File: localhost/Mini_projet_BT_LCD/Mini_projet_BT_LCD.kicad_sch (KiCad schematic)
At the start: 9 parts

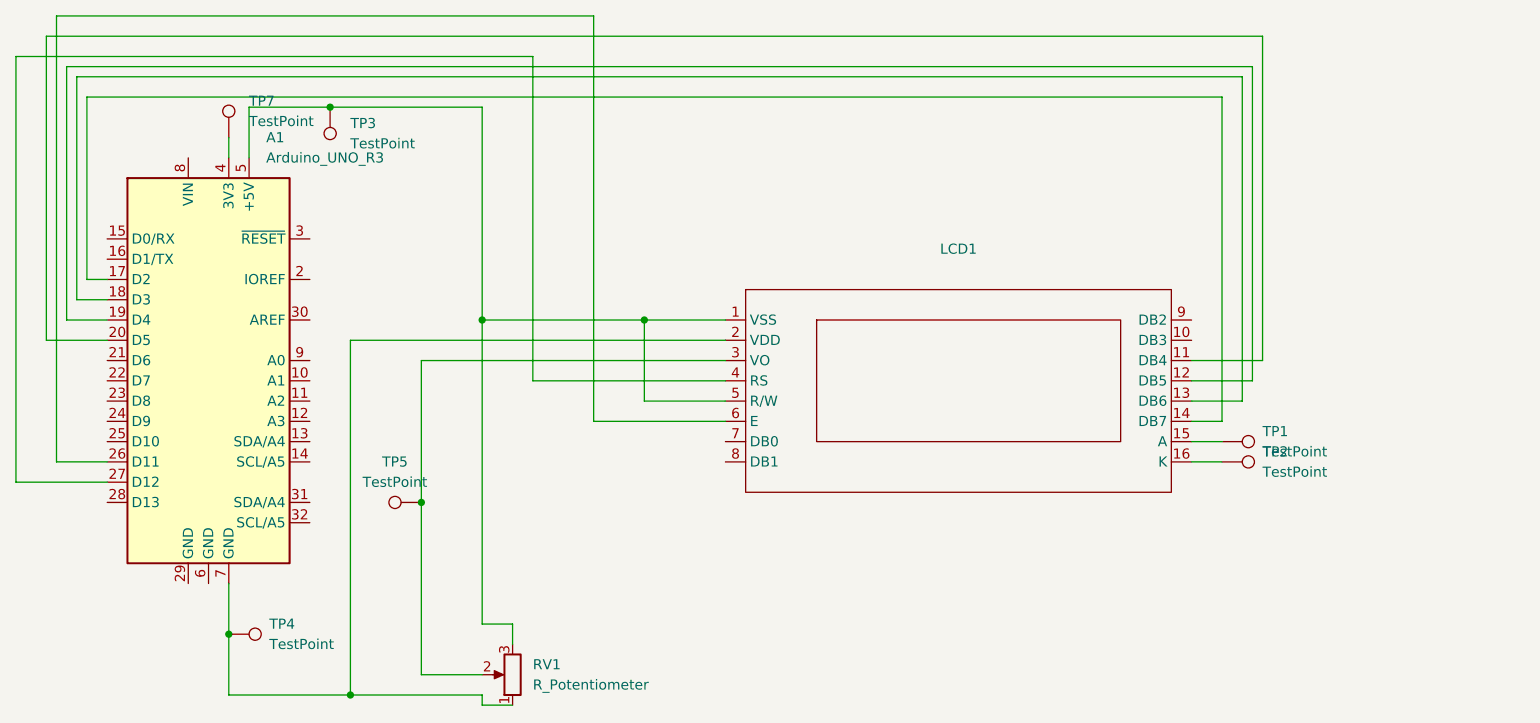
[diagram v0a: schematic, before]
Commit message: Mise à jour 2
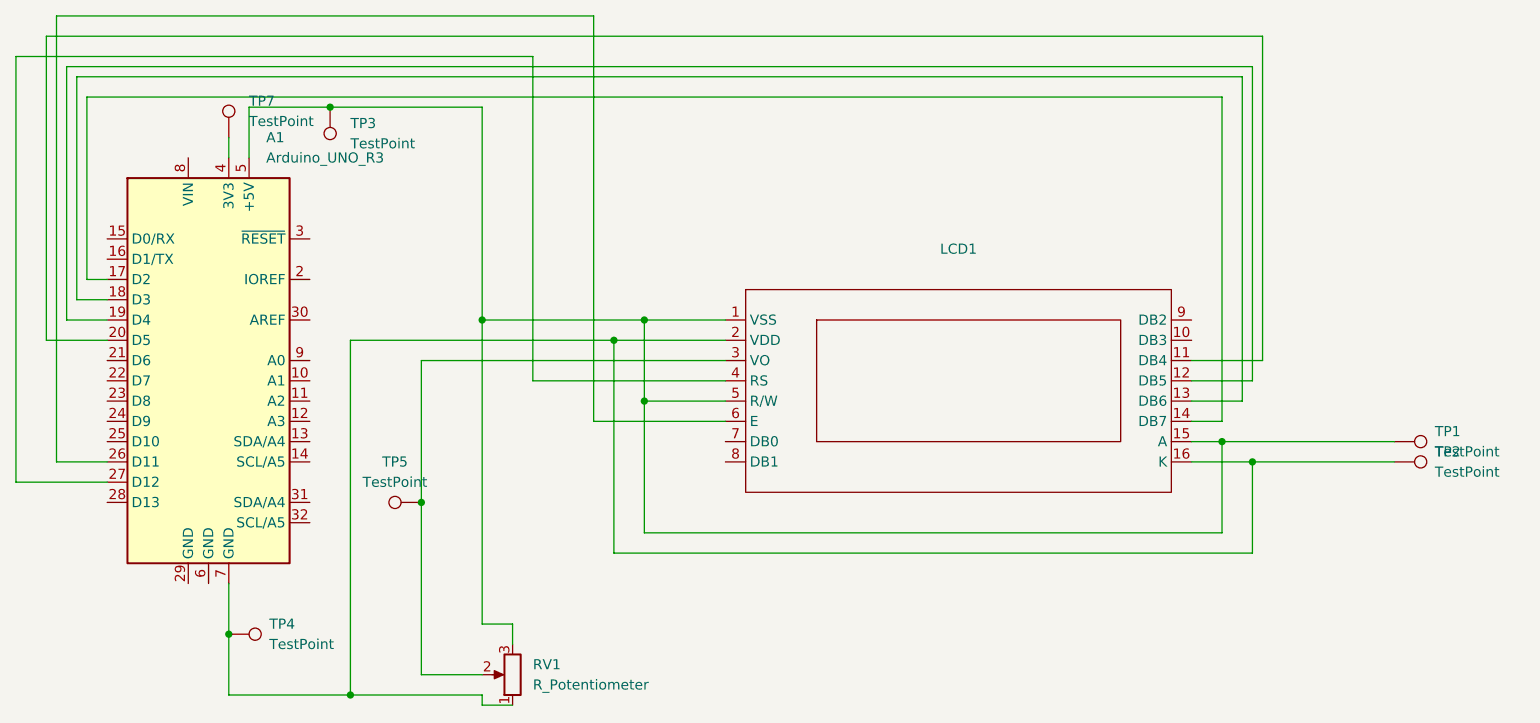
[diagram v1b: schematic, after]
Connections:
- net at A1.7 (GND), LCD1.2 (VDD), RV1.1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: now also LCD1.16 (K), TP2.1
- net at A1.5 (+5V), LCD1.1 (VSS), LCD1.5 (R/W)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: now also LCD1.15 (A), TP1.1
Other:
- moved on the sheet: TP1, TP2
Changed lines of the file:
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@@
+	)
+	(junction
+		(at 193.04 85.09)
+		(diameter 0)
+		(color 0 0 0 0)
 	)
 	(junction
@@
 	)
 	(junction
+		(at 116.84 72.39)
+		(diameter 0)
+		(color 0 0 0 0)
+	)
+	(junction
 		(at 92.71 92.71)
+		(diameter 0)
+		(color 0 0 0 0)
+	)
+	(junction
+		(at 120.65 80.01)
 		(diameter 0)
 		(color 0 0 0 0)
@@
 	)
 	(junction
+		(at 196.85 87.63)
+		(diameter 0)
+		(color 0 0 0 0)
+	)
+	(junction
 		(at 81.28 43.18)
 		(diameter 0)
@@
 	(wire
 		(pts
-			(xy 83.82 72.39) (xy 130.81 72.39)
+			(xy 196.85 87.63) (xy 214.63 87.63)
+		)
+		(stroke
+			(width 0)
+			(type default)
+		)
+	)
+	(wire
+		(pts
+			(xy 120.65 96.52) (xy 120.65 80.01)
+		)
+		(stroke
+			(width 0)
+			(type default)
+			(color 255 0 4 1)
+		)
+	)
+	(wire
+		(pts
+			(xy 83.82 72.39) (xy 116.84 72.39)
 		)
 		(stroke
@@
 	(wire
 		(pts
+			(xy 193.04 96.52) (xy 120.65 96.52)
+		)
+		(stroke
+			(width 0)
+			(type default)
+			(color 255 0 4 1)
+		)
+	)
+	(wire
+		(pts
 			(xy 130.81 80.01) (xy 120.65 80.01)
 		)
@@
 	(wire
 		(pts
+			(xy 196.85 99.06) (xy 116.84 99.06)
+		)
+		(stroke
+			(width 0)
+			(type default)
+			(color 0 0 0 1)
+		)
+	)
+	(wire
+		(pts
 			(xy 49.53 67.31) (xy 53.34 67.31)
 		)
@@
 	(wire
 		(pts
-			(xy 189.23 87.63) (xy 193.04 87.63)
+			(xy 189.23 87.63) (xy 196.85 87.63)
 		)
 		(stroke
@@
 	(wire
 		(pts
+			(xy 116.84 72.39) (xy 130.81 72.39)
+		)
+		(stroke
+			(width 0)
+			(type default)
+			(color 0 0 0 1)
+		)
+	)
+	(wire
+		(pts
+			(xy 196.85 87.63) (xy 196.85 99.06)
+		)
+		(stroke
+			(width 0)
+			(type default)
+			(color 0 0 0 1)
+		)
+	)
+	(wire
+		(pts
+			(xy 116.84 99.06) (xy 116.84 72.39)
+		)
+		(stroke
+			(width 0)
+			(type default)
+			(color 0 0 0 1)
+		)
+	)
+	(wire
+		(pts
 			(xy 83.82 116.84) (xy 68.58 116.84)
 		)
@@
 	(wire
 		(pts
+			(xy 193.04 85.09) (xy 214.63 85.09)
+		)
+		(stroke
+			(width 0)
+			(type default)
+		)
+	)
+	(wire
+		(pts
 			(xy 196.85 38.1) (xy 48.26 38.1)
 		)
@@
 			(type default)
 			(color 0 0 0 1)
+		)
+	)
+	(wire
+		(pts
+			(xy 193.04 85.09) (xy 193.04 96.52)
+		)
+		(stroke
+			(width 0)
+			(type default)
+			(color 255 0 4 1)
 		)
 	)
@@
 	(symbol
 		(lib_id "Connector:TestPoint")
-		(at 193.04 87.63 270)
+		(at 214.63 87.63 270)
 		(unit 1)
 		(exclude_from_sim no)
@@
 		(fields_autoplaced yes)
 		(property "Reference" "TP2"
-			(at 198.12 86.3599 90)
+			(at 219.71 86.3599 90)
 			(effects
 				(font
@@
 		)
 		(property "Value" "TestPoint"
-			(at 198.12 88.8999 90)
+			(at 219.71 88.8999 90)
 			(effects
 				(font
@@
 		)
 		(property "Footprint" "Connector_PinHeader_1.00mm:PinHeader_1x01_P1.00mm_Vertical"
-			(at 193.04 92.71 0)
+			(at 214.63 92.71 0)
 			(effects
 				(font
@@
 		)
 		(property "Datasheet" "~"
-			(at 193.04 92.71 0)
+			(at 214.63 92.71 0)
 			(effects
 				(font
@@
 		)
 		(property "Description" "test point"
-			(at 193.04 87.63 0)
+			(at 214.63 87.63 0)
 			(effects
 				(font
@@
 	(symbol
 		(lib_id "Connector:TestPoint")
-		(at 193.04 85.09 270)
+		(at 214.63 85.09 270)
 		(unit 1)
 		(exclude_from_sim no)
@@
 		(fields_autoplaced yes)
 		(property "Reference" "TP1"
-			(at 198.12 83.8199 90)
+			(at 219.71 83.8199 90)
 			(effects
 				(font
@@
 		)
 		(property "Value" "TestPoint"
-			(at 198.12 86.3599 90)
+			(at 219.71 86.3599 90)
 			(effects
 				(font
@@
 		)
 		(property "Footprint" "Connector_PinHeader_1.00mm:PinHeader_1x01_P1.00mm_Vertical"
-			(at 193.04 90.17 0)
+			(at 214.63 90.17 0)
 			(effects
 				(font
@@
 		)
 		(property "Datasheet" "~"
-			(at 193.04 90.17 0)
+			(at 214.63 90.17 0)
 			(effects
 				(font
@@
 		)
 		(property "Description" "test point"
-			(at 193.04 85.09 0)
-			(effects
-				(font
+			(at 214.63 85.09 0)
+			(effects
+				(font
